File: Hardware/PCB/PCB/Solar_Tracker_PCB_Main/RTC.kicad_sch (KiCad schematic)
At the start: 10 parts, among them IC4 PCF2131TFY

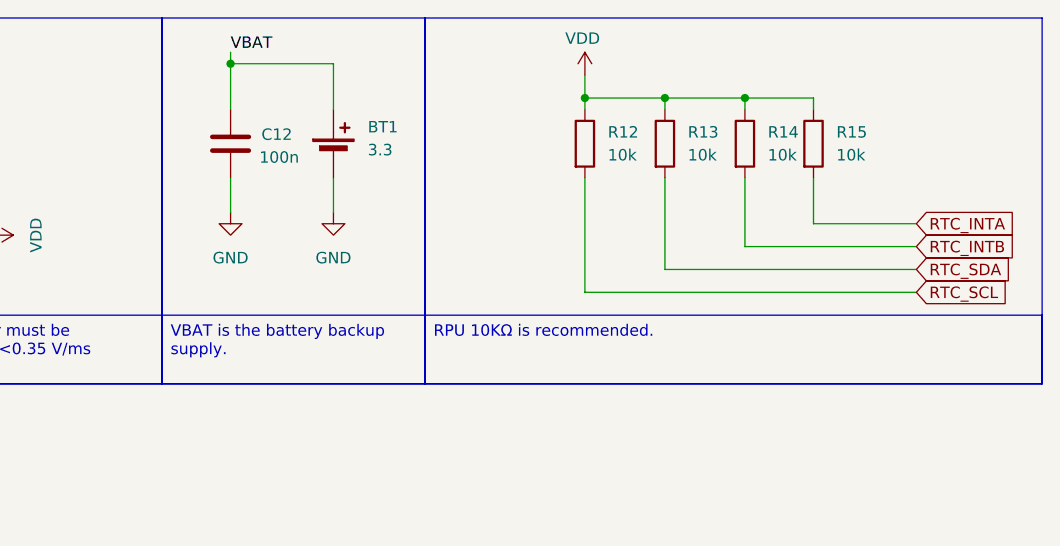
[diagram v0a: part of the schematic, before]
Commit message: Actualizacion Main pcb
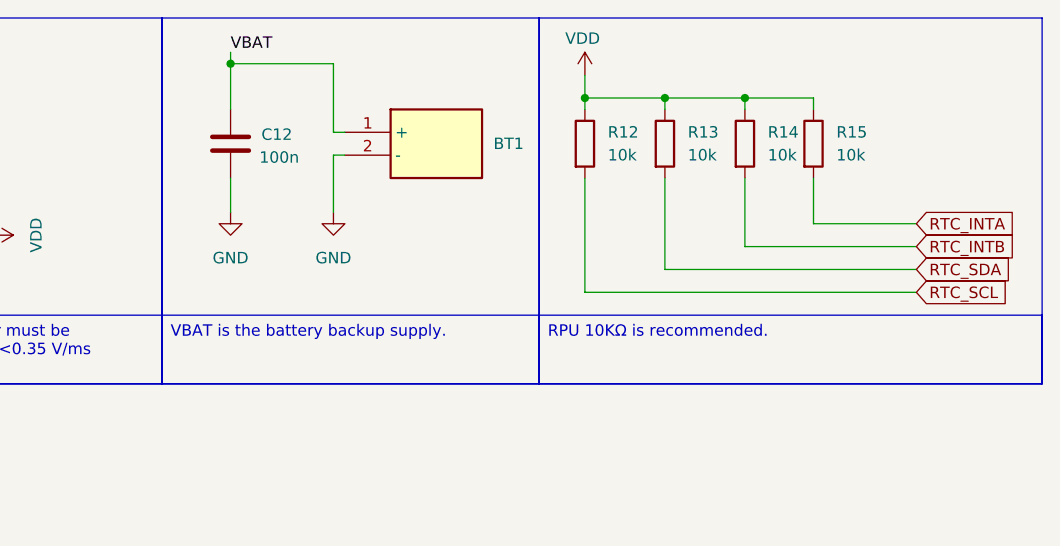
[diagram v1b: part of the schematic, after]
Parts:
- removed BT1: 3.3, symbol Device:Battery_Cell
- added BT1: BAT-HLD-013-SMT-TR, BAT-HLD:BATHLD013SMTTR, symbol BAT-HLD-013-SMT-TR:BAT-HLD-013-SMT-TR
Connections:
- net GND: now also BT1.2 (-)
- net VBAT: now also BT1.1 (+)
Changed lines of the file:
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@@
 	(rectangle
 		(start 66.04 12.7)
-		(end 95.25 53.34)
+		(end 107.95 53.34)
 		(stroke
 			(width 0)
@@
 	)
 	(rectangle
-		(start 95.25 12.7)
+		(start 107.95 12.7)
 		(end 163.83 53.34)
 		(stroke
@@
 		(exclude_from_sim no)
 		(at 66.04 45.72 0)
-		(size 29.21 7.62)
+		(size 41.91 7.62)
 		(margins 0.9525 0.9525 0.9525 0.9525)
 		(stroke
@@
 	(text_box "RPU 10KΩ is recommended."
 		(exclude_from_sim no)
-		(at 95.25 45.72 0)
-		(size 68.58 7.62)
+		(at 107.95 45.72 0)
+		(size 55.88 7.62)
 		(margins 0.9525 0.9525 0.9525 0.9525)
 		(stroke
@@
 	(wire
 		(pts
-			(xy 85.09 30.48) (xy 85.09 34.29)
+			(xy 85.09 27.94) (xy 85.09 34.29)
 		)
 		(stroke
@@
 	(wire
 		(pts
+			(xy 86.36 27.94) (xy 85.09 27.94)
+		)
+		(stroke
+			(width 0)
+			(type default)
+		)
+	)
+	(wire
+		(pts
 			(xy 121.92 40.64) (xy 149.86 40.64)
 		)
@@
 	(wire
 		(pts
-			(xy 85.09 17.78) (xy 85.09 22.86)
-		)
-		(stroke
-			(width 0)
-			(type default)
-		)
-	)
-	(wire
-		(pts
 			(xy 130.81 22.86) (xy 130.81 21.59)
 		)
@@
 	(wire
 		(pts
+			(xy 85.09 17.78) (xy 85.09 25.4)
+		)
+		(stroke
+			(width 0)
+			(type default)
+		)
+	)
+	(wire
+		(pts
 			(xy 130.81 38.1) (xy 149.86 38.1)
 		)
@@
 		(pts
 			(xy 49.53 86.36) (xy 63.5 86.36)
+		)
+		(stroke
+			(width 0)
+			(type default)
+		)
+	)
+	(wire
+		(pts
+			(xy 86.36 25.4) (xy 85.09 25.4)
 		)
 		(stroke
@@
 	)
 	(symbol
+		(lib_id "BAT-HLD-013-SMT-TR:BAT-HLD-013-SMT-TR")
+		(at 86.36 25.4 0)
+		(unit 1)
+		(exclude_from_sim no)
+		(in_bom yes)
+		(on_board yes)
+		(dnp no)
+		(fields_autoplaced yes)
+		(property "Reference" "BT1"
+			(at 102.87 26.6699 0)
+			(effects
+				(font
+					(size 1.27 1.27)
+				)
+				(justify left)
+			)
+		)
+		(property "Value" "BAT-HLD-013-SMT-TR"
+			(at 102.87 27.9399 0)
+			(effects
+				(font
+					(size 1.27 1.27)
+				)
+				(justify left)
+				(hide yes)
+			)
+		)
+		(property "Footprint" "BAT-HLD:BATHLD013SMTTR"
+			(at 102.87 120.32 0)
+			(effects
+				(font
+					(size 1.27 1.27)
+				)
+				(justify left top)
+				(hide yes)
+			)
+		)
+		(property "Datasheet" "https://www.te.com/en/product-BAT-HLD-013-SMT-TR.html"
+			(at 102.87 220.32 0)
+			(effects
+				(font
+					(size 1.27 1.27)
+				)
+				(justify left top)
+				(hide yes)
+			)
+		)
+		(property "Description" "CR2032 Battery Holder, 1 Position, Horizontal, Nickel (Ni)"
+			(at 86.36 25.4 0)
+			(effects
+				(font
+					(size 1.27 1.27)
+				)
+				(hide yes)
+			)
+		)
+		(property "Height" "6.5"
+			(at 102.87 420.32 0)
+			(effects
+				(font
+					(size 1.27 1.27)
+				)
+				(justify left top)
+				(hide yes)
+			)
+		)
+		(property "Mouser Part Number" "712-BAT-HLD-013SMTTR"
+			(at 102.87 520.32 0)
+			(effects
+				(font
+					(size 1.27 1.27)
+				)
+				(justify left top)
+				(hide yes)
+			)
+		)
+		(property "Mouser Price/Stock" "https://www.mouser.co.uk/ProductDetail/TE-Connectivity-Linx-Technologies/BAT-HLD-013-SMT-TR?qs=4ASt3YYao0UKhYWrBts7tw%3D%3D"
+			(at 102.87 620.32 0)
+			(effects
+				(font
+					(size 1.27 1.27)
+				)
+				(justify left top)
+				(hide yes)
+			)
+		)
+		(property "Manufacturer_Name" "TE Connectivity"
+			(at 102.87 720.32 0)
+			(effects
+				(font
+					(size 1.27 1.27)
+				)
+				(justify left top)
+				(hide yes)
+			)
+		)
+		(property "Manufacturer_Part_Number" "BAT-HLD-013-SMT-TR"
+			(at 102.87 820.32 0)
+			(effects
+				(font
+					(size 1.27 1.27)
+				)
+				(justify left top)
+				(hide yes)
+			)
+		)
+		(pin "1"
+		)
+		(pin "2"
+		)
+		(instances
+			(project ""
+				(path "/99b6ddd9-7ffe-4c85-972a-e0f594a166d4/f065d8bf-f34b-491d-8721-3ae145af2fae"
+					(reference "BT1")
+					(unit 1)
+				)
+			)
+		)
+	)
+	(symbol
 		(lib_id "Device:R")
 		(at 113.03 26.67 0)
@@
 					(unit 1)
 				)
-			)
-		)
-	)
-	(symbol
-		(lib_id "Device:Battery_Cell")
-		(at 85.09 27.94 0)
-		(unit 1)
-		(exclude_from_sim no)
-		(in_bom yes)
-		(on_board yes)
-		(dnp no)
-		(fields_autoplaced yes)
-		(property "Reference" "BT1"
-			(at 88.9 24.8284 0)
-			(effects
-				(font
-					(size 1.27 1.27)
-				)
-				(justify left)
-			)
-		)
-		(property "Value" "3.3"
-			(at 88.9 27.3684 0)
-			(effects
-				(font
-					(size 1.27 1.27)
-				)
-				(justify left)
-			)
-		)
-		(property "Footprint" ""
-			(at 85.09 26.416 90)
-			(effects
-				(font
-					(size 1.27 1.27)
-				)
-				(hide yes)
-			)
-		)
-		(property "Datasheet" "~"
-			(at 85.09 26.416 90)
-			(effects
-				(font
-					(size 1.27 1.27)
-				)
-				(hide yes)
-			)
-		)
-		(property "Description" "Single-cell battery"
-			(at 85.09 27.94 0)
-			(effects
-				(font
-					(size 1.27 1.27)
-				)
-				(hide yes)
-			)
-		)
-		(property "Sim.Device" "V"
-			(at 85.09 27.94 0)
-			(effects
-				(font
-					(size 1.27 1.27)
-				)
-				(hide yes)
-			)
-		)
-		(property "Sim.Type" "DC"
-			(at 85.09 27.94 0)
-			(effects
-				(font
-					(size 1.27 1.27)
-				)
-				(hide yes)
-			)
-		)
-		(property "Sim.Pins" "1=+ 2=-"
-			(at 85.09 27.94 0)
-			(effects
-				(font
-					(size 1.27 1.27)
-				)
-				(hide yes)
-			)
-		)
-		(pin "2"
-		)
-		(pin "1"
-		)
-		(instances
-			(project ""
-				(path "/99b6ddd9-7ffe-4c85-972a-e0f594a166d4/f065d8bf-f34b-491d-8721-3ae145af2fae"
-					(reference "BT1")
-					(unit 1)
-				)
